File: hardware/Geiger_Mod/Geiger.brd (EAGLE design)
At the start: 52.1 x 30.5 mm, 20 parts, among them Q1 KSP44, Q2 2N3904, X1 GM-tube

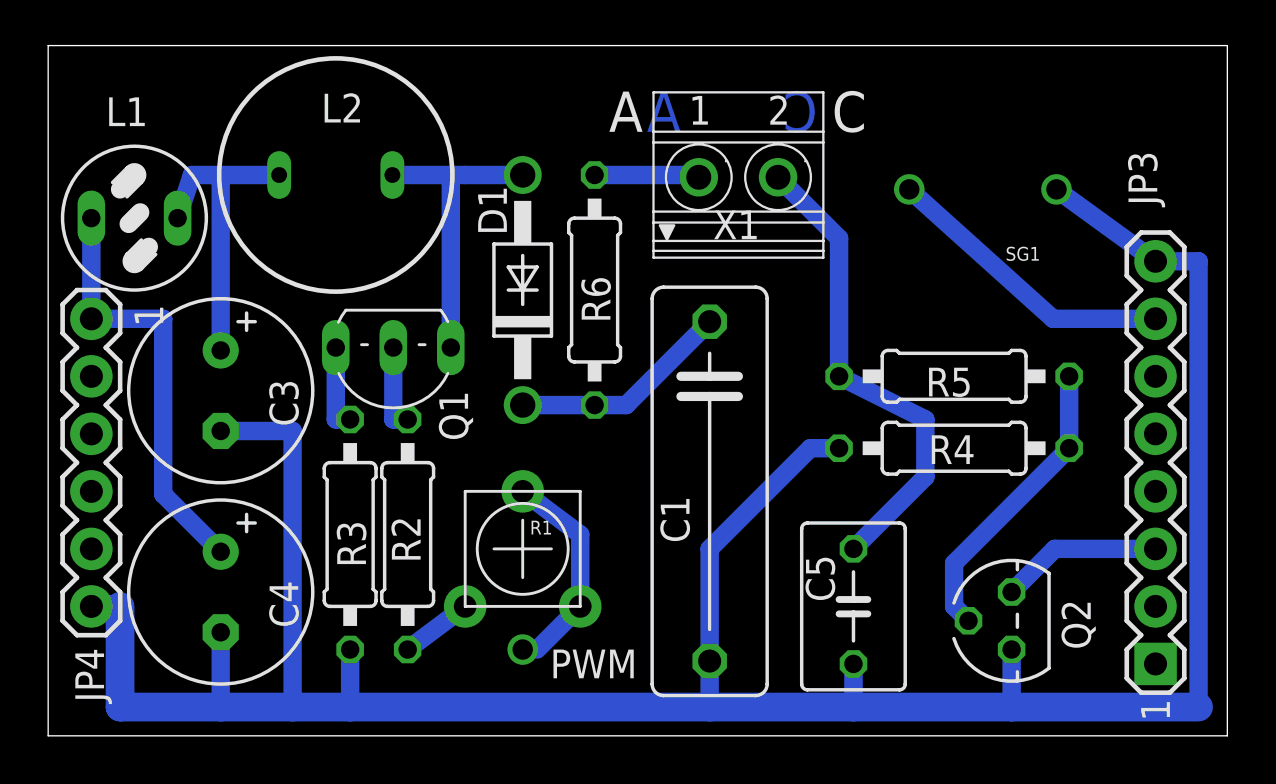
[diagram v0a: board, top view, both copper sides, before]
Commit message: layout changes
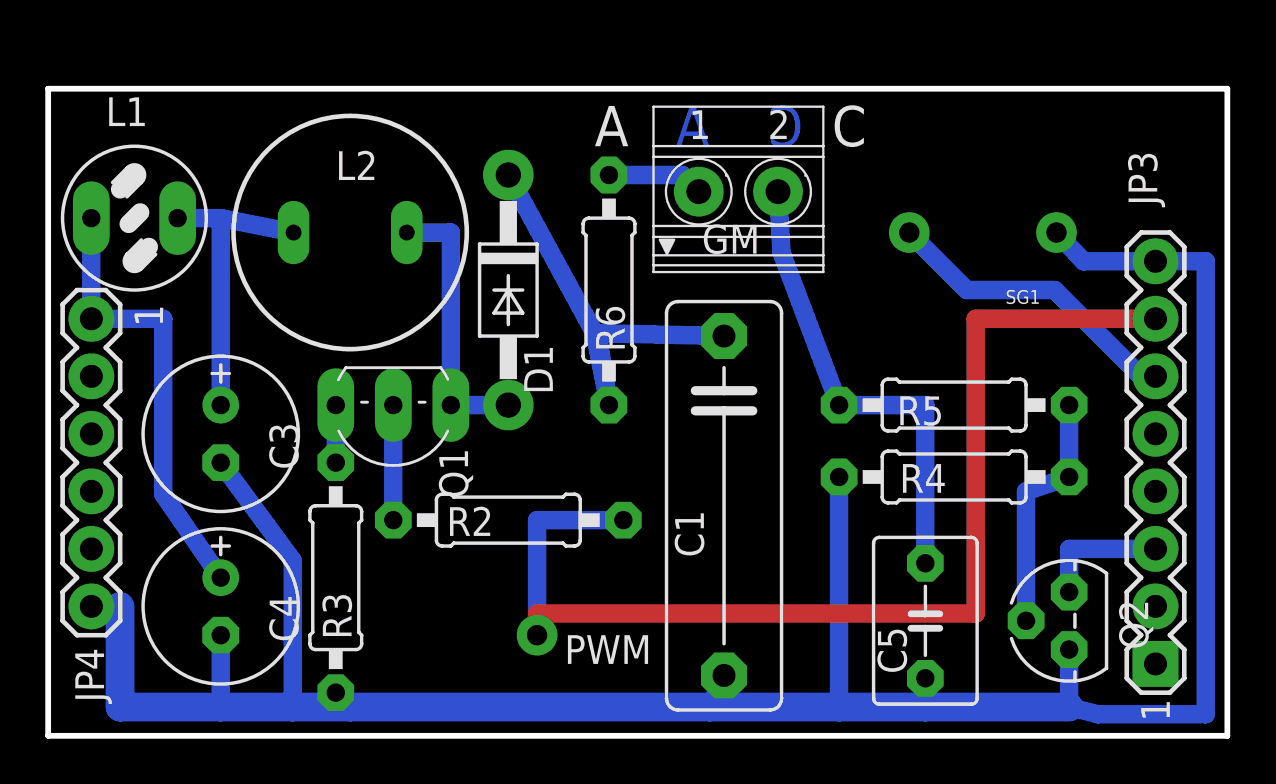
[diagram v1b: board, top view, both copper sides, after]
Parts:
- removed R1: 1K, SparkFun-Electromechanical:TRIM_POT_PTH
- removed X1: GM-tube, con-phoenix-350:1751248
- added GM: GM-tube, con-phoenix-350:1751248
- C3, C4: device rcl:E3,5-8 -> rcl:E2,5-7
- moved R2 4.49 mm to (26.7, 32.4), turned to 0 degrees
- moved C5 3.24 mm to (45.1, 27.9)
- moved L2 2.62 mm to (19.7, 45.1)
- moved Q1 2.54 mm to (21.6, 36.2)
- moved Q2 2.54 mm to (51.4, 27.9)
- moved R3 2.01 mm to (19.1, 29.8)
- moved C3 1.91 mm to (14.0, 36.2)
- moved SG1 1.91 mm to (47.6, 45.1)
- moved R4 1.27 mm to (46.4, 34.3)
- moved R5 1.27 mm to (46.4, 37.5)
- moved PWM 0.90 mm to (27.9, 27.3)
- moved C1 0.90 mm to (36.2, 33.0)
- moved C4 0.64 mm to (14.0, 28.6)
- moved D1 0.63 mm to (26.7, 42.5), turned to 270 degrees
- moved R6 0.63 mm to (31.1, 42.5)
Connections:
- removed net N$14: JP3.7, SG1.+
- removed net N$15: PWM.1, R1.2, R1.3
- new net N$3: JP3.6, SG1.+
- net N$1: now also JP3.7, PWM.1; no longer R1.1
- net N$10: now also GM.1; no longer X1.1
- net N$13: now also GM.2; no longer X1.2
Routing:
- net N$1: track 3.17 -> 50.2 mm
- net N$3: track 0.00 -> 13.5 mm
- net N$14: track 13.1 -> 0.00 mm
- net N$9: track 9.78 -> 20.0 mm
- net N$15: track 9.68 -> 0.00 mm
- net GND: track 121.2 -> 112.9 mm
- net N$11: track 13.2 -> 10.9 mm
- net RESET: track 7.14 -> 5.72 mm
- net N$2: track 3.81 -> 5.08 mm
- net N$6: track 13.4 -> 12.1 mm
- net N$5: track 3.81 -> 2.54 mm
- net +5V: track 19.0 -> 19.8 mm
- net N$13: track 21.2 -> 20.7 mm
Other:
- board size 52.1 x 30.5 mm -> 52.1 x 28.6 mm
